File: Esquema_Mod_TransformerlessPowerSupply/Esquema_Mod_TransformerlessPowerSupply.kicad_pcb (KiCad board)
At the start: 2 copper layers, 18 parts, among them J1 Screw_Terminal_01x02, J2 Screw_Terminal_01x02, U1 LM7805_TO220

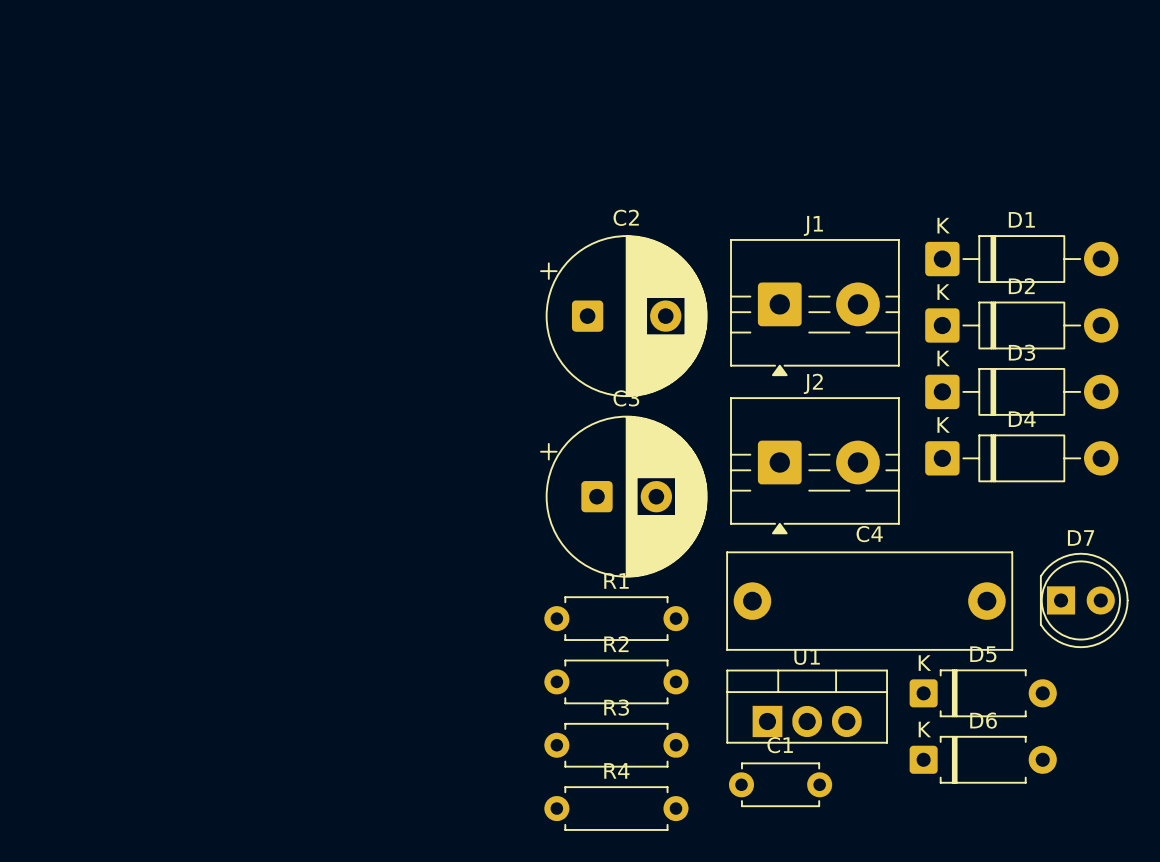
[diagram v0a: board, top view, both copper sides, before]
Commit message: [ADD] some projects
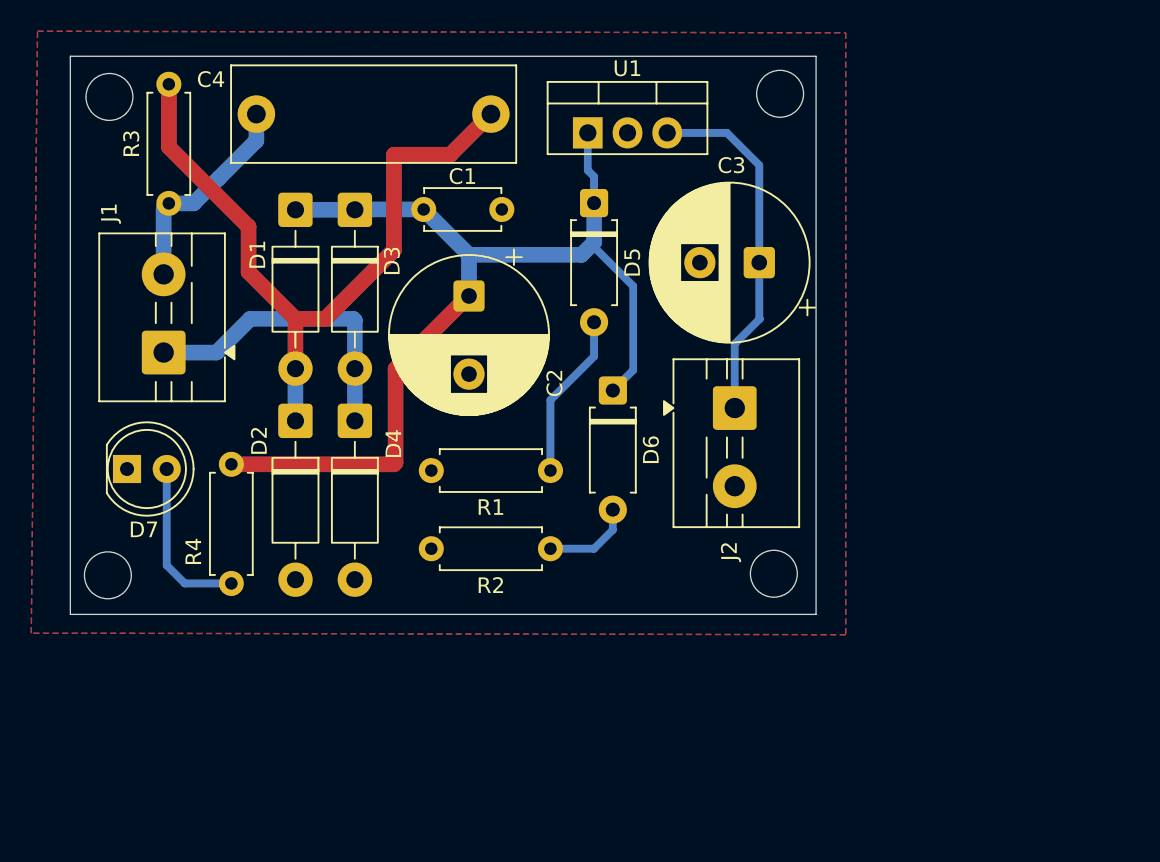
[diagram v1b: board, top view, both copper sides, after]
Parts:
- moved D7 60.3 mm to (139.5, 102.3)
- moved C4 44.5 mm to (147.8, 79.6)
- moved R3 42.6 mm to (142.2, 85.3), turned to 90 degrees
- moved C1 42.0 mm to (158.5, 85.7)
- moved D2 41.8 mm to (150.3, 99.2), turned to -90 degrees
- moved D1 41.5 mm to (150.3, 85.7), turned to -90 degrees
- moved J1 39.5 mm to (141.9, 94.8), turned to 90 degrees
- moved U1 39.4 mm to (169.0, 80.8)
- moved D3 39.3 mm to (154.1, 85.7), turned to -90 degrees
- moved D5 37.8 mm to (169.4, 85.3), turned to -90 degrees
- moved D4 37.7 mm to (154.1, 99.2), turned to -90 degrees
- moved D6 30.9 mm to (170.6, 97.3), turned to -90 degrees
- moved R4 30.3 mm to (146.2, 102.0), turned to -90 degrees
- moved C3 18.2 mm to (180.0, 89.1), turned to 180 degrees
- moved R1 9.48 mm to (166.6, 102.4), turned to 180 degrees
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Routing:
- net Net-(D1-K): track 0.00 -> 64.7 mm
- net Net-(D1-A): track 0.00 -> 46.4 mm
- net /5V: track 0.00 -> 23.0 mm
- net Net-(D3-A): track 0.00 -> 19.6 mm
- net Net-(J1-Pin_2): track 0.00 -> 13.6 mm
- net Net-(D7-A): track 0.00 -> 10.8 mm
- net Net-(D5-A): track 0.00 -> 10.6 mm
- net Net-(D6-A): track 0.00 -> 5.79 mm
- added copper zone on B.Cu, net GND
- added copper zone on F.Cu, net GND
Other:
- board outline added: 47.7 x 35.7 mm
